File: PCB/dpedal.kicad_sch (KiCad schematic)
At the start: 26 parts, among them J1 USB_C_Receptacle_USB2.0, J2 Conn_02x10_Counter_Clockwise, J3 Conn_ARM_JTAG_SWD_10, J4 Conn_01x05, SW1 SW_Push, SW10 SW_Push, SW2 SW_Push, SW3 SW_Push, SW4 SW_Push, SW5 RESET, SW6 FLASH, SW7 SW_Push, SW8 SW_Push, SW9 SW_Push, U1 STM32F072C8Tx, U2 LDO

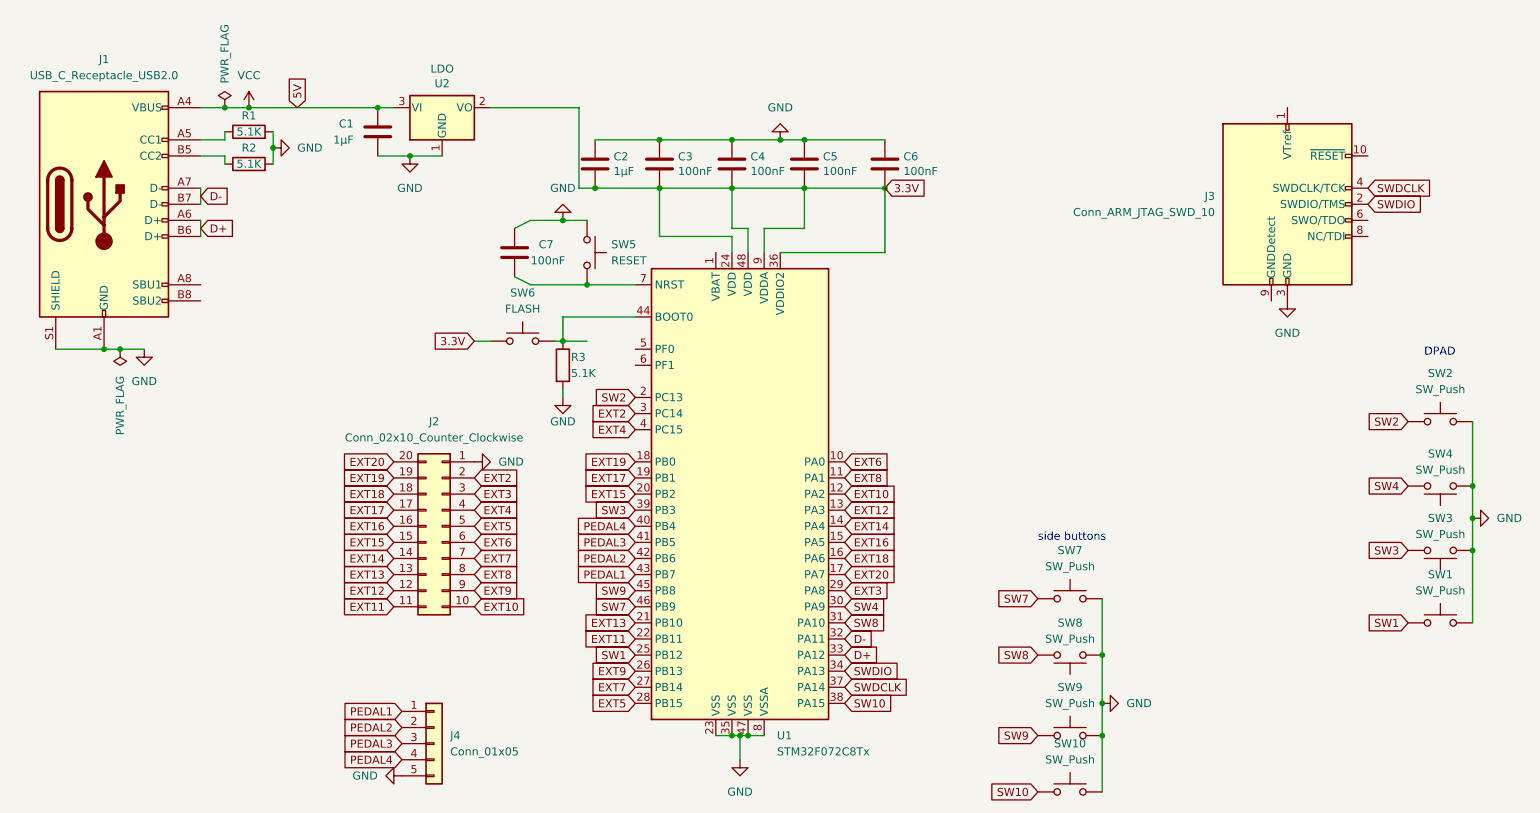
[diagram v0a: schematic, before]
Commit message: Update symbols/footprints
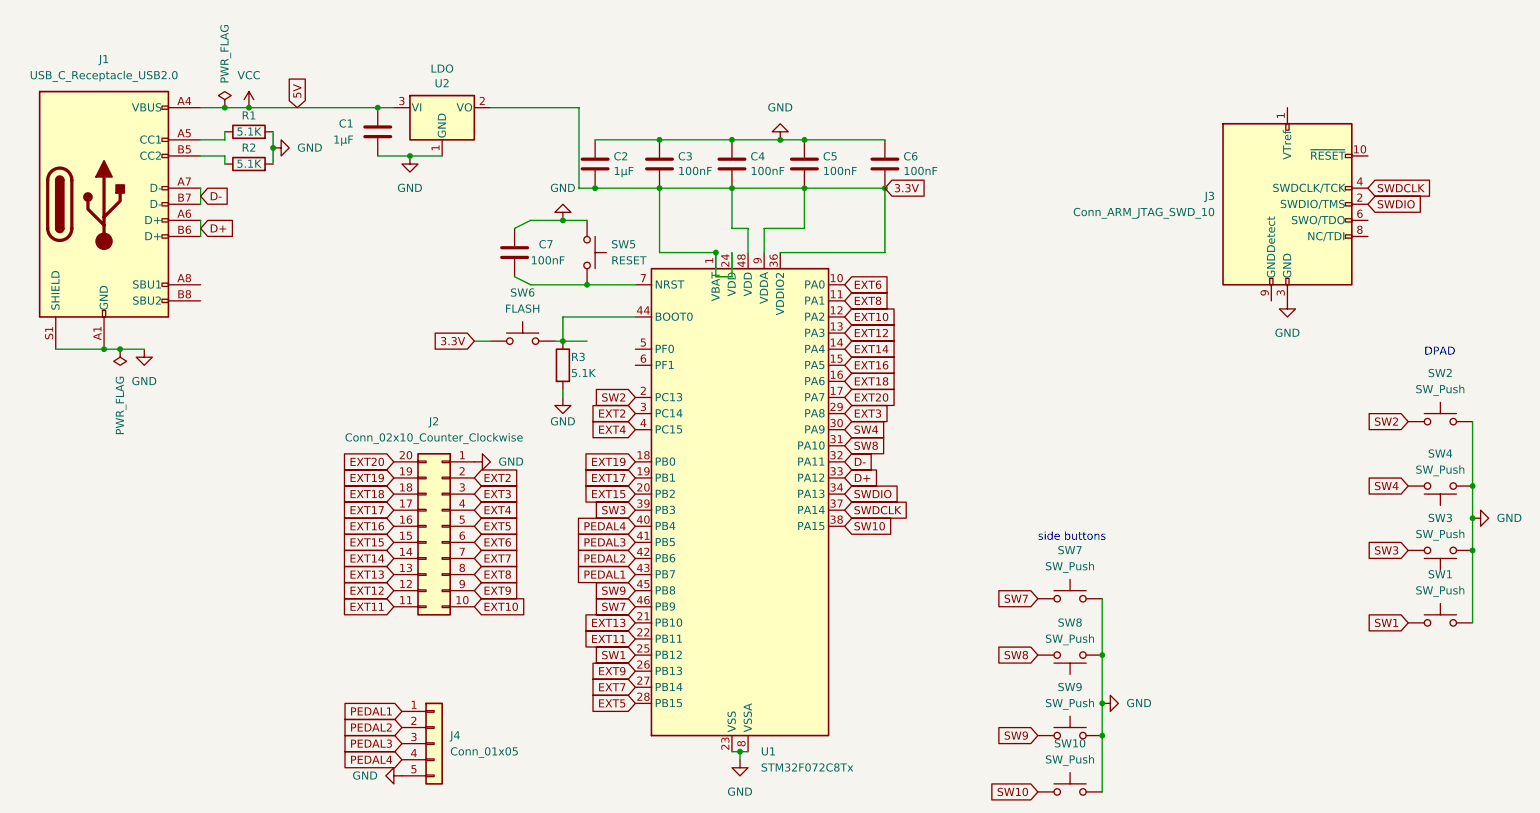
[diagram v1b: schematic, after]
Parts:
- U2: footprint Package_TO_SOT_SMD:SOT-23 -> Package_TO_SOT_SMD:SOT-23-3; symbol Regulator_Linear:MCP1703A-3302_SOT23 -> Regulator_Linear:XC6206PxxxMR
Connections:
- net 3.3V: now also U1.1 (VBAT)
